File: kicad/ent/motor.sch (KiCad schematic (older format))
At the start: 28 parts, among them J10 Conn_01x02_Male, J11 Conn_01x02_Male, J12 Barrel_Jack, J13 Conn_01x12_Male, J14 Conn_01x12_Male, J8 Conn_01x02_Male, J9 Conn_01x02_Male, U4 IFX9201SGAUMA1, U5 IFX9201SGAUMA1, U6 IFX9201SGAUMA1, U7 IFX9201SGAUMA1

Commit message: begin pcb
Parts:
- J10, J11, J8, J9: footprint (none) -> Connector_JST:JST_SFH_SM02B-SFHRS-TF_1x02-1MP_P4.20mm_Horizontal
- J12: footprint (none) -> PJ-082BH:CUI_PJ-082BH; symbol Connector:Barrel_Jack -> ent-rescue:PJ-082BH
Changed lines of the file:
@@
 EESchema Schematic File Version 4
-LIBS:ent-cache
-EELAYER 29 0
+EELAYER 30 0
 EELAYER END
 $Descr A4 11693 8268
@@
 F 0 "J8" H 1758 2481 50  0000 C CNN
 F 1 "Conn_01x02_Male" H 1758 2390 50  0000 C CNN
-F 2 "" H 1650 2300 50  0001 C CNN
+F 2 "Connector_JST:JST_SFH_SM02B-SFHRS-TF_1x02-1MP_P4.20mm_Horizontal" H 1650 2300 50  0001 C CNN
 F 3 "~" H 1650 2300 50  0001 C CNN
 	1    1650 2300
@@
 F 0 "J9" H 1758 3631 50  0000 C CNN
 F 1 "Conn_01x02_Male" H 1758 3540 50  0000 C CNN
-F 2 "" H 1650 3450 50  0001 C CNN
+F 2 "Connector_JST:JST_SFH_SM02B-SFHRS-TF_1x02-1MP_P4.20mm_Horizontal" H 1650 3450 50  0001 C CNN
 F 3 "~" H 1650 3450 50  0001 C CNN
 	1    1650 3450
@@
 F 0 "J10" H 1808 4631 50  0000 C CNN
 F 1 "Conn_01x02_Male" H 1808 4540 50  0000 C CNN
-F 2 "" H 1700 4450 50  0001 C CNN
+F 2 "Connector_JST:JST_SFH_SM02B-SFHRS-TF_1x02-1MP_P4.20mm_Horizontal" H 1700 4450 50  0001 C CNN
 F 3 "~" H 1700 4450 50  0001 C CNN
 	1    1700 4450
@@
 F 0 "J11" H 1858 5681 50  0000 C CNN
 F 1 "Conn_01x02_Male" H 1858 5590 50  0000 C CNN
-F 2 "" H 1750 5500 50  0001 C CNN
+F 2 "Connector_JST:JST_SFH_SM02B-SFHRS-TF_1x02-1MP_P4.20mm_Horizontal" H 1750 5500 50  0001 C CNN
 F 3 "~" H 1750 5500 50  0001 C CNN
 	1    1750 5500
@@
 M4OUT1
 Text GLabel 4150 4800 2    50   Input ~ 0
-M2OUT2
+M3OUT2
 $Comp
 L Device:D_Zener D1
@@
 	4400 1200 4800 1200
 $Comp
-L Connector:Barrel_Jack J12
+L ent-rescue:PJ-082BH J12
 U 1 1 5E661C20
 P 5750 1200
-F 0 "J12" H 5807 1525 50  0000 C CNN
-F 1 "Barrel_Jack" H 5807 1434 50  0000 C CNN
-F 2 "" H 5800 1160 50  0001 C CNN
+F 0 "J12" H 5750 1650 50  0000 C CNN
+F 1 "Barrel_Jack" H 5750 1550 50  0000 C CNN
+F 2 "PJ-082BH:CUI_PJ-082BH" H 5800 1160 50  0001 C CNN
 F 3 "~" H 5800 1160 50  0001 C CNN
 	1    5750 1200
@@
 L power:+12V #PWR067
 U 1 1 5E6687C4
-P 6050 1100
-F 0 "#PWR067" H 6050 950 50  0001 C CNN
-F 1 "+12V" V 6065 1228 50  0000 L CNN
-F 2 "" H 6050 1100 50  0001 C CNN
-F 3 "" H 6050 1100 50  0001 C CNN
-	1    6050 1100
+P 6250 1000
+F 0 "#PWR067" H 6250 850 50  0001 C CNN
+F 1 "+12V" V 6265 1128 50  0000 L CNN
+F 2 "" H 6250 1000 50  0001 C CNN
+F 3 "" H 6250 1000 50  0001 C CNN
+	1    6250 1000
 	0    1    1    0
 $EndComp
@@
 L power:GND #PWR?
 U 1 1 5E669336
-P 6050 1300
+P 6250 1400
 AR Path="/5E669336" Ref="#PWR?"  Part="1"
 AR Path="/5E68BD2A/5E669336" Ref="#PWR068"  Part="1"
-F 0 "#PWR068" H 6050 1050 50  0001 C CNN
-F 1 "GND" H 6055 1127 50  0000 C CNN
-F 2 "" H 6050 1300 50  0001 C CNN
-F 3 "" H 6050 1300 50  0001 C CNN
-	1    6050 1300
+F 0 "#PWR068" H 6250 1150 50  0001 C CNN
+F 1 "GND" H 6255 1227 50  0000 C CNN
+F 2 "" H 6250 1400 50  0001 C CNN
+F 3 "" H 6250 1400 50  0001 C CNN
+	1    6250 1400
 	1    0    0    -1
 $EndComp
@@
 M3OUT2
 Text GLabel 2600 5800 0    50   Input ~ 0
-M3OUT1
+M4OUT1
 $Comp
 L power:GND #PWR?
@@
 $EndComp
 Text GLabel 2000 5800 0    50   Input ~ 0
-M3OUT2
+M4OUT2
+$Comp
+L power:GND #PWR?
+U 1 1 5E659BDE
+P 6250 1200
+AR Path="/5E659BDE" Ref="#PWR?"  Part="1"
+AR Path="/5E68BD2A/5E659BDE" Ref="#PWR069"  Part="1"
+F 0 "#PWR069" H 6250 950 50  0001 C CNN
+F 1 "GND" H 6255 1027 50  0000 C CNN
+F 2 "" H 6250 1200 50  0001 C CNN
+F 3 "" H 6250 1200 50  0001 C CNN
+	1    6250 1200
+	1    0    0    -1
+$EndComp
 $EndSCHEMATC

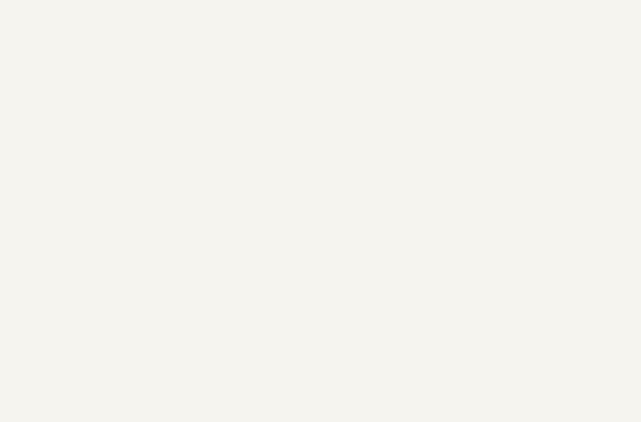
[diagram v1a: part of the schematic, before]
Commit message: pcb done
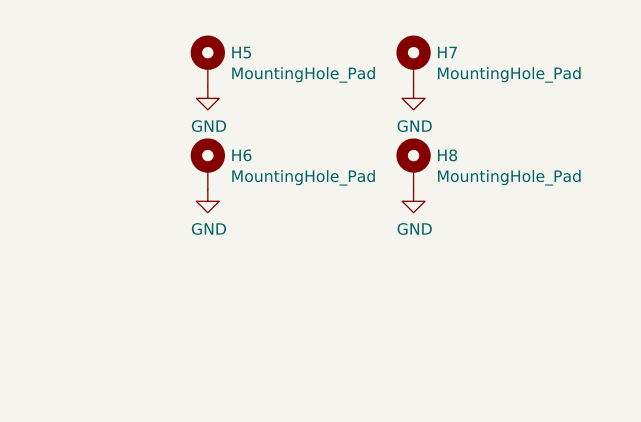
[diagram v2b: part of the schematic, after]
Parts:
- added H5, H6, H7, H8: MountingHole_Pad, MountingHole:MountingHole_2.2mm_M2_Pad, symbol Mechanical:MountingHole_Pad
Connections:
- net GND: now also H5.1, H6.1, H7.1, H8.1
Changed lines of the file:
@@
+	1    0    0    -1
+$EndComp
+$Comp
+L Mechanical:MountingHole_Pad H?
+U 1 1 5E723063
+P 10100 900
+AR Path="/5E723063" Ref="H?"  Part="1"
+AR Path="/5E68BD2A/5E723063" Ref="H7"  Part="1"
+F 0 "H7" H 10200 949 50  0000 L CNN
+F 1 "MountingHole_Pad" H 10200 858 50  0000 L CNN
+F 2 "MountingHole:MountingHole_2.2mm_M2_Pad" H 10100 900 50  0001 C CNN
+F 3 "~" H 10100 900 50  0001 C CNN
+	1    10100 900
+	1    0    0    -1
+$EndComp
+$Comp
+L Mechanical:MountingHole_Pad H?
+U 1 1 5E723069
+P 10100 1350
+AR Path="/5E723069" Ref="H?"  Part="1"
+AR Path="/5E68BD2A/5E723069" Ref="H8"  Part="1"
+F 0 "H8" H 10200 1399 50  0000 L CNN
+F 1 "MountingHole_Pad" H 10200 1308 50  0000 L CNN
+F 2 "MountingHole:MountingHole_2.2mm_M2_Pad" H 10100 1350 50  0001 C CNN
+F 3 "~" H 10100 1350 50  0001 C CNN
+	1    10100 1350
+	1    0    0    -1
+$EndComp
+$Comp
+L Mechanical:MountingHole_Pad H?
+U 1 1 5E72306F
+P 9200 900
+AR Path="/5E72306F" Ref="H?"  Part="1"
+AR Path="/5E68BD2A/5E72306F" Ref="H5"  Part="1"
+F 0 "H5" H 9300 949 50  0000 L CNN
+F 1 "MountingHole_Pad" H 9300 858 50  0000 L CNN
+F 2 "MountingHole:MountingHole_2.2mm_M2_Pad" H 9200 900 50  0001 C CNN
+F 3 "~" H 9200 900 50  0001 C CNN
+	1    9200 900
+	1    0    0    -1
+$EndComp
+$Comp
+L Mechanical:MountingHole_Pad H?
+U 1 1 5E723075
+P 9200 1350
+AR Path="/5E723075" Ref="H?"  Part="1"
+AR Path="/5E68BD2A/5E723075" Ref="H6"  Part="1"
+F 0 "H6" H 9300 1399 50  0000 L CNN
+F 1 "MountingHole_Pad" H 9300 1308 50  0000 L CNN
+F 2 "MountingHole:MountingHole_2.2mm_M2_Pad" H 9200 1350 50  0001 C CNN
+F 3 "~" H 9200 1350 50  0001 C CNN
+	1    9200 1350
+	1    0    0    -1
+$EndComp
+$Comp
+L power:GND #PWR?
+U 1 1 5E72307B
+P 10100 1000
+AR Path="/5E72307B" Ref="#PWR?"  Part="1"
+AR Path="/5E68BD2A/5E72307B" Ref="#PWR0106"  Part="1"
+F 0 "#PWR0106" H 10100 750 50  0001 C CNN
+F 1 "GND" H 10105 827 50  0000 C CNN
+F 2 "" H 10100 1000 50  0001 C CNN
+F 3 "" H 10100 1000 50  0001 C CNN
+	1    10100 1000
+	1    0    0    -1
+$EndComp
+$Comp
+L power:GND #PWR?
+U 1 1 5E723081
+P 10100 1450
+AR Path="/5E723081" Ref="#PWR?"  Part="1"
+AR Path="/5E68BD2A/5E723081" Ref="#PWR0107"  Part="1"
+F 0 "#PWR0107" H 10100 1200 50  0001 C CNN
+F 1 "GND" H 10105 1277 50  0000 C CNN
+F 2 "" H 10100 1450 50  0001 C CNN
+F 3 "" H 10100 1450 50  0001 C CNN
+	1    10100 1450
+	1    0    0    -1
+$EndComp
+$Comp
+L power:GND #PWR?
+U 1 1 5E723087
+P 9200 1450
+AR Path="/5E723087" Ref="#PWR?"  Part="1"
+AR Path="/5E68BD2A/5E723087" Ref="#PWR0108"  Part="1"
+F 0 "#PWR0108" H 9200 1200 50  0001 C CNN
+F 1 "GND" H 9205 1277 50  0000 C CNN
+F 2 "" H 9200 1450 50  0001 C CNN
+F 3 "" H 9200 1450 50  0001 C CNN
+	1    9200 1450
+	1    0    0    -1
+$EndComp
+$Comp
+L power:GND #PWR?
+U 1 1 5E72308D
+P 9200 1000
+AR Path="/5E72308D" Ref="#PWR?"  Part="1"
+AR Path="/5E68BD2A/5E72308D" Ref="#PWR0109"  Part="1"
+F 0 "#PWR0109" H 9200 750 50  0001 C CNN
+F 1 "GND" H 9205 827 50  0000 C CNN
+F 2 "" H 9200 1000 50  0001 C CNN
+F 3 "" H 9200 1000 50  0001 C CNN
+	1    9200 1000
 	1    0    0    -1
 $EndComp
